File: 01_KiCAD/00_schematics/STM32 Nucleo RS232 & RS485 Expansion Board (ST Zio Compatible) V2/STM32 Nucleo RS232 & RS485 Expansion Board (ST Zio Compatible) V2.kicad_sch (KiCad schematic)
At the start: 0 parts

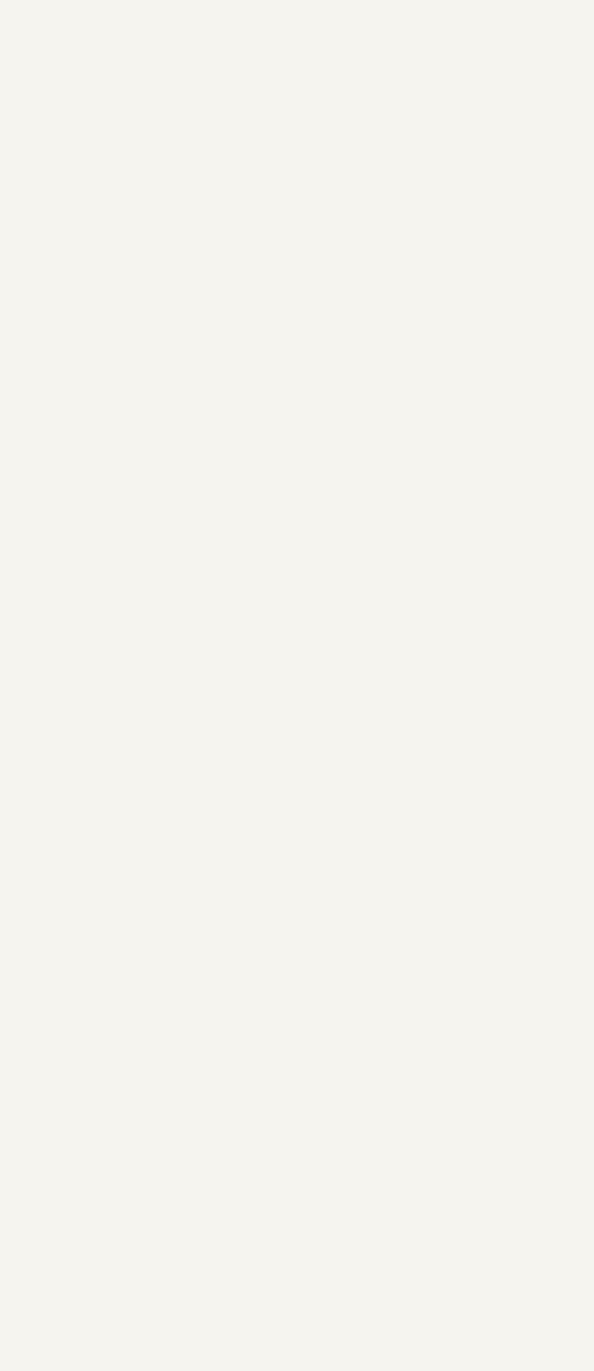
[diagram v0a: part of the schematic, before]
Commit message: Added half-duplex jumpers
Addres jumpers for hardware RS485 half-duplex configuration combining signals A(Y) & B(Z). Finalising testpoints and added 3D models for each test-point color.
-Green = logic side
-Blue = connector side
Made some minor changed to layout for test signals clarification (THVD4431 sheet)
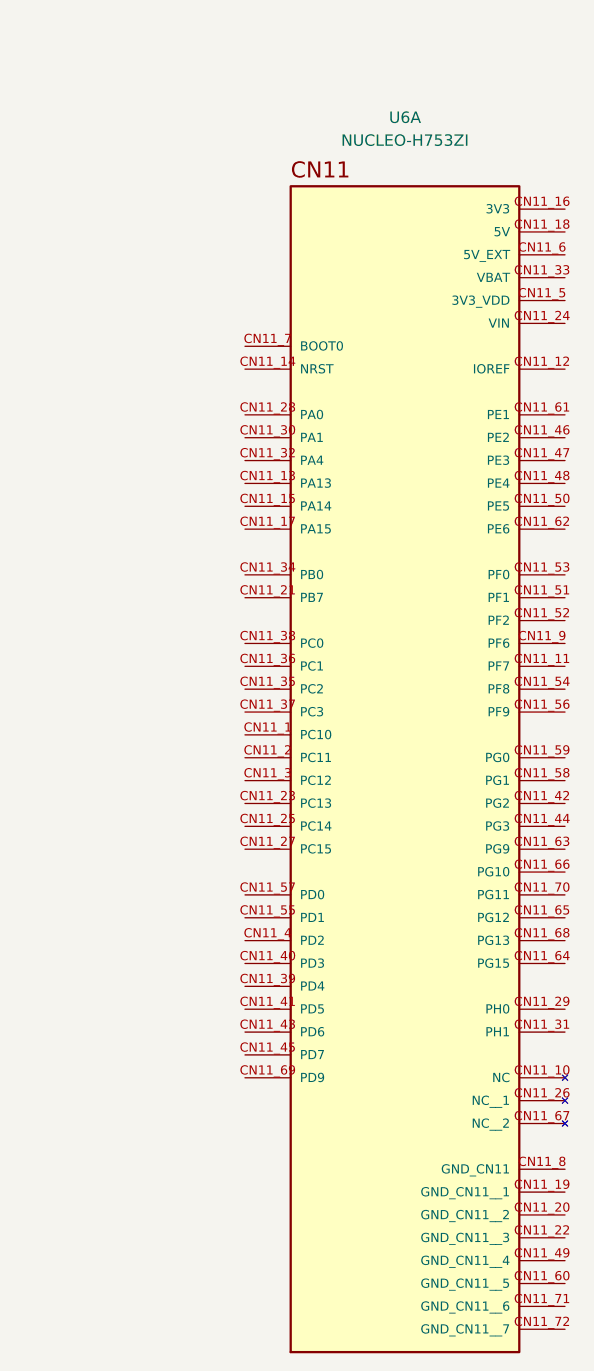
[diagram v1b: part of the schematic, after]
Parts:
- added U6: NUCLEO-H753ZI, NUCLEO-H753ZI:MODULE_NUCLEO-H753ZI, symbol NUCLEO-H753ZI:NUCLEO-H753ZI

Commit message: Finalizing PCB Design
Finalizing track routing on PCB and run DRC. Made some minor silkscreen adjustments.
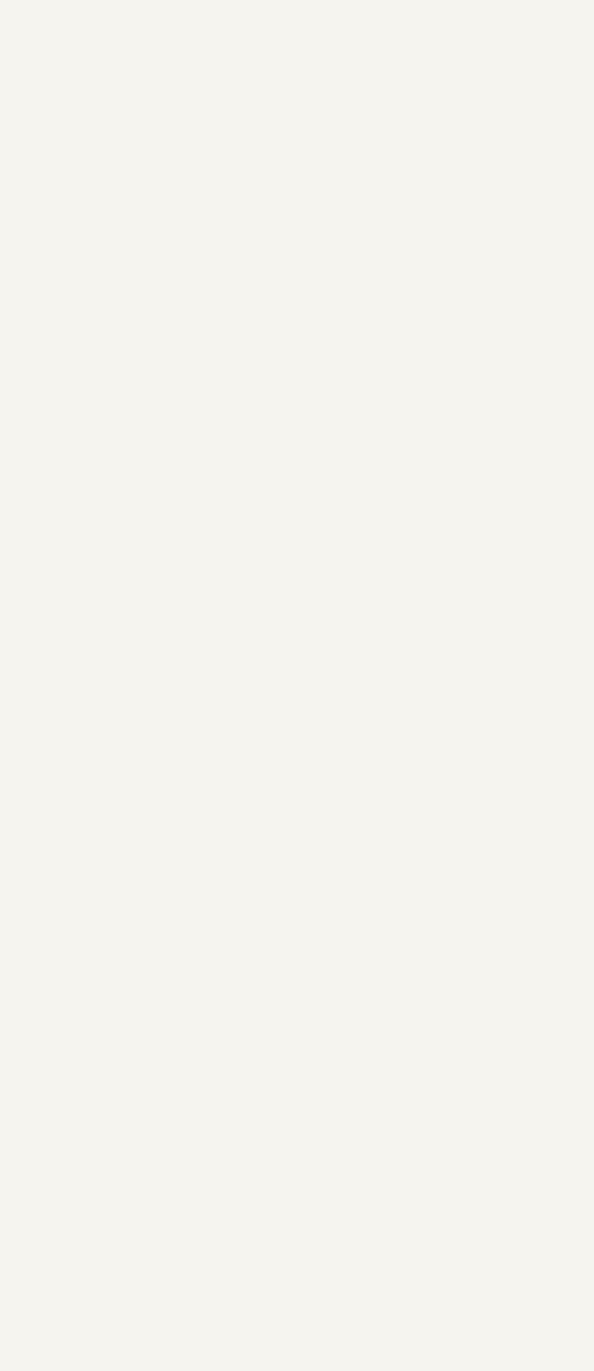
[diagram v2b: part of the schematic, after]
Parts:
- removed U6: NUCLEO-H753ZI, NUCLEO-H753ZI:MODULE_NUCLEO-H753ZI, symbol NUCLEO-H753ZI:NUCLEO-H753ZI
